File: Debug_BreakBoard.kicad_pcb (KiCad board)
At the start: 2 copper layers, 100 x 26 mm, 70 parts, among them J1 FFC2A32-12-T, J10 Conn_01x03_Pin, J11 Conn_01x03_Pin, J12 Conn_01x03_Pin, J13 Conn_01x03_Pin, J14 Conn_01x03_Pin, J15 Conn_01x03_Pin, J16 Conn_01x03_Pin, J17 Conn_01x02_Pin, J2 Conn_02x12_Counter_Clockwise, J3 Conn_01x03_Pin, J4 Conn_02x12_Counter_Clockwise, J5 Conn_01x03_Pin, J6 Conn_01x03_Pin, J7 Conn_01x03_Pin, J8 Conn_02x12_Counter_Clockwise, J9 Conn_01x03_Pin, P1 USB4125-GF-A-0190, SW1 SW_Push, SW10 SW_Push, SW11 SW_Push, SW12 SW_Push, SW2 SW_Push, SW3 SW_Push, SW4 SW_Push, SW5 SW_Push, SW6 SW_Push, SW7 SW_Push, SW8 SW_Push, SW9 SW_Push, U1 TLV6001UIDBVR, U10 TLV6001UIDBVR, U11 TLV6001UIDBVR, U12 TLV6001UIDBVR, U2 TLV6001UIDBVR, U3 TLV6001UIDBVR, U4 TLV6001UIDBVR, U5 TLV6001UIDBVR, U6 TLV6001UIDBVR, U7 TLV6001UIDBVR, U8 TLV6001UIDBVR, U9 TLV6001UIDBVR

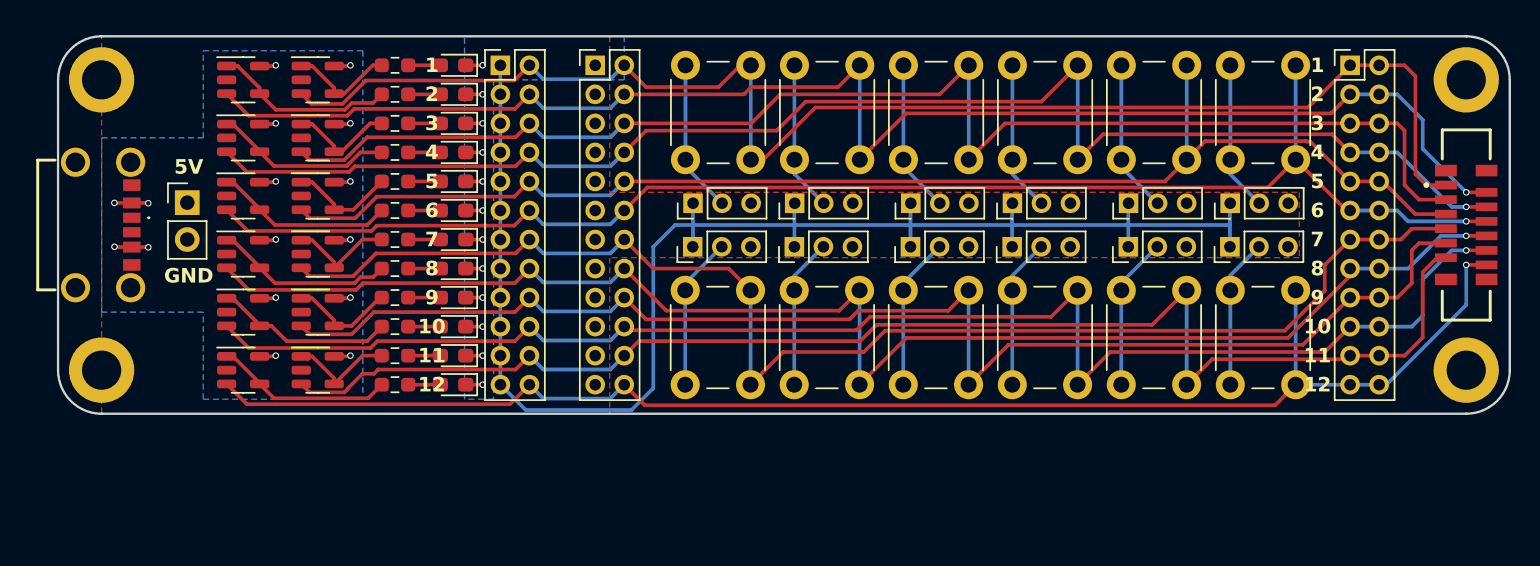
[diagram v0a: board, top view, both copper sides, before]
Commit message: bom
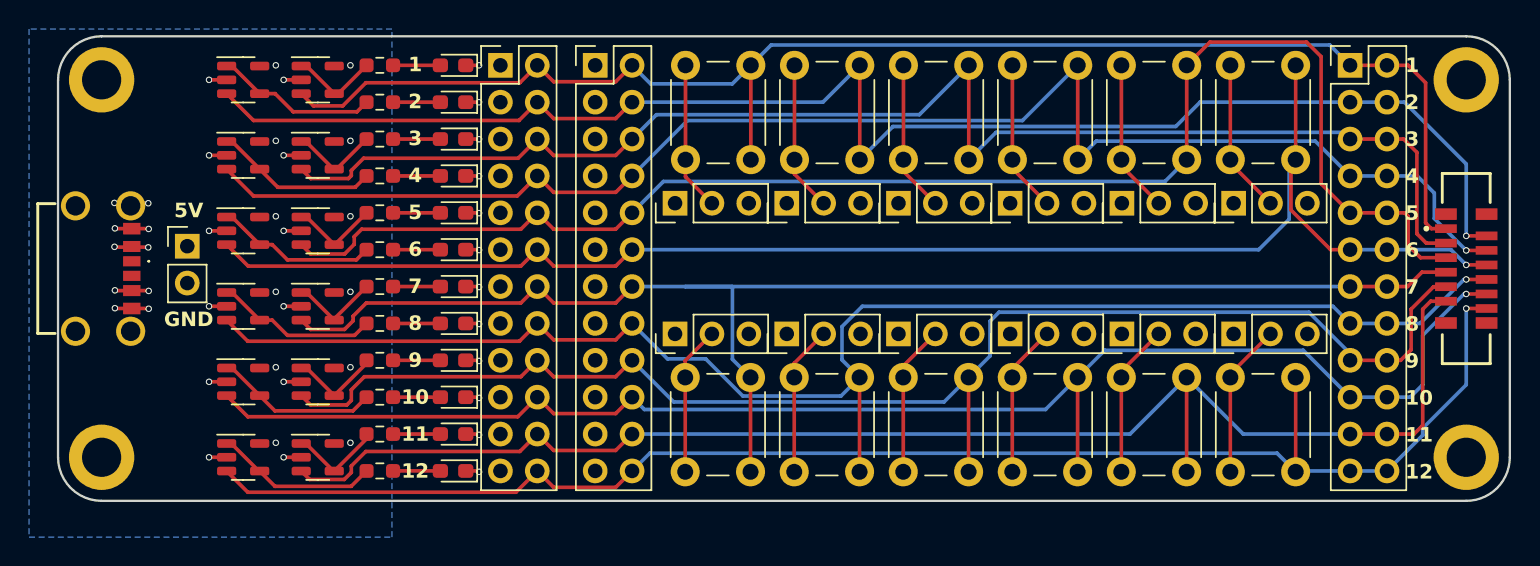
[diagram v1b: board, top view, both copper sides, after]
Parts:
- J10, J11, J12, J13, J14, J15, J16, J3, J5, J6, J7, J9: footprint Connector_PinHeader_2.00mm:PinHeader_1x03_P2.00mm_Vertical -> Connector_PinHeader_2.54mm:PinHeader_1x03_P2.54mm_Vertical
- J2, J4, J8: footprint Connector_PinHeader_2.00mm:PinHeader_2x12_P2.00mm_Vertical -> Connector_PinHeader_2.54mm:PinHeader_2x12_P2.54mm_Vertical
- moved J3 6.12 mm to (139.5, 67.5)
- moved J6 6.06 mm to (154.9, 67.5)
- moved R12 6.03 mm to (119.2, 76.9)
- moved J5 6.02 mm to (147.2, 67.5)
- moved J9 6.02 mm to (170.3, 67.5)
- moved J10 6.01 mm to (178.0, 67.5)
- moved J7 6.00 mm to (162.6, 67.5)
- moved H2 6.00 mm to (100.0, 76.0)
- moved H4 6.00 mm to (194.0, 76.0)
- moved SW1 6.00 mm to (140.2, 77.0)
- moved SW2 6.00 mm to (147.7, 77.0)
- moved SW3 6.00 mm to (155.2, 77.0)
- moved SW4 6.00 mm to (162.7, 77.0)
- moved SW5 6.00 mm to (170.2, 77.0)
- moved SW6 6.00 mm to (177.8, 77.0)
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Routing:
- net VDD: track 101.8 -> 0.00 mm
- net GND: track 14.0 -> 32.7 mm, vias 12 -> 30
- net P5V0: track 18.3 -> 4.69 mm
- net /5: track 90.7 -> 102.7 mm
- net /6: track 98.2 -> 105.5 mm
- net /11: track 94.6 -> 99.8 mm
- net /9: track 94.2 -> 98.8 mm
- net /8: track 101.1 -> 105.5 mm
- net /7: track 94.4 -> 98.4 mm
- net /12: track 101.4 -> 104.5 mm
- net /1: track 97.3 -> 100.3 mm
- net /2: track 102.0 -> 104.9 mm
- net /4: track 100.5 -> 103.4 mm
- net /3: track 94.5 -> 97.2 mm
- net /10: track 101.5 -> 103.7 mm
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- added copper zone on In1.Cu, net GND
- added copper zone on In2.Cu, net VDD
- removed copper zone on B.Cu, net GND
- removed copper zone on F.Cu, net GND
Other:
- board size 100 x 26 mm -> 100 x 32 mm
- copper layers 2 -> 4
